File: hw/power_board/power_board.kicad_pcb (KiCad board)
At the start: 2 copper layers, 61 x 106.7 mm, 44 parts, among them P1 SIGNAL_IN, P10 SPINDLE_C_BLOCK, P11 POWER_IN, P12 SPINDLE_PWR_OUT, P2 SPINDLE_REALY, P3 SOFT_RELAY, P4 DIS_RELAY, P5 STEPPER_RELAY, P6 STOP_RELAY, P7 SPINDLE_RPWR_IN, P8 SOFT_RELAY_OUT, P9 DIS_RELAY_OUT, Q1 Q_NMOS_GDS, Q2 Q_NMOS_GDS, Q3 Q_NMOS_GDS, Q4 Q_NMOS_GDS, Q5 Q_NMOS_GDS

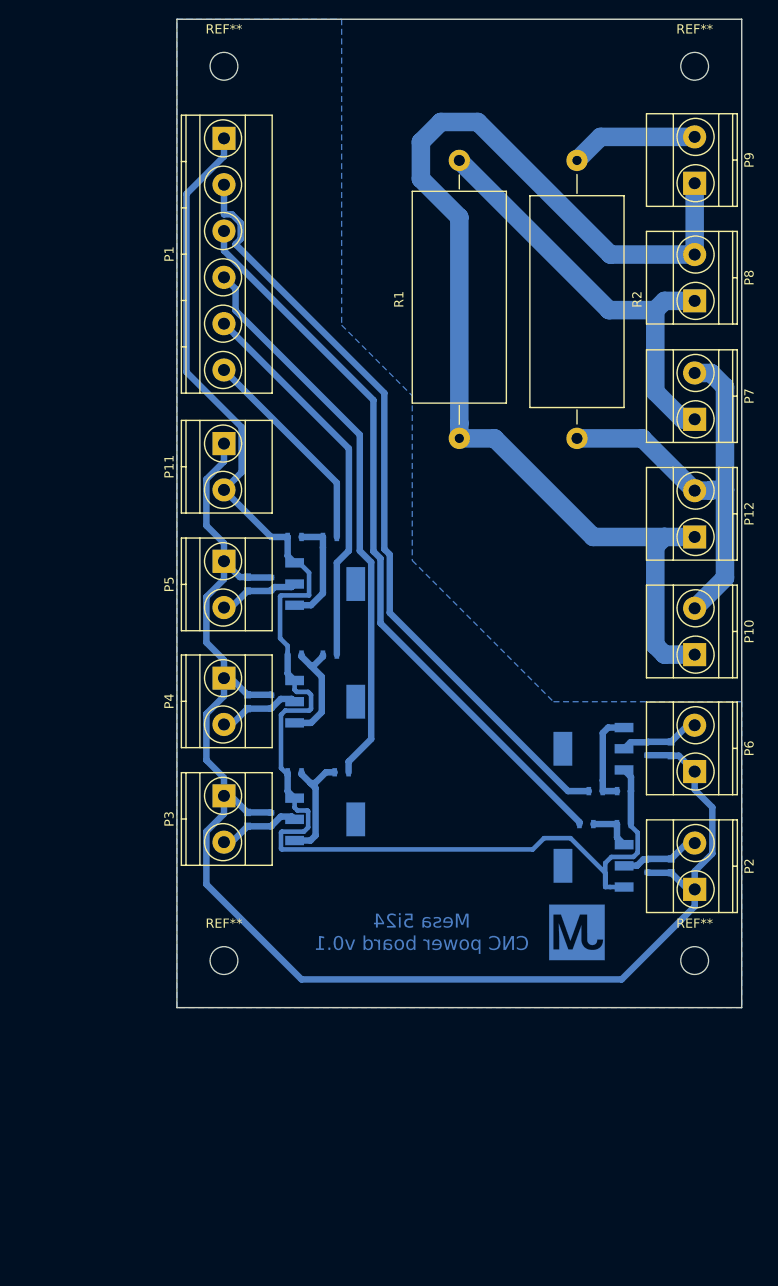
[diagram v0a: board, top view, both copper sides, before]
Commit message: Tweak power and breakout boards a little
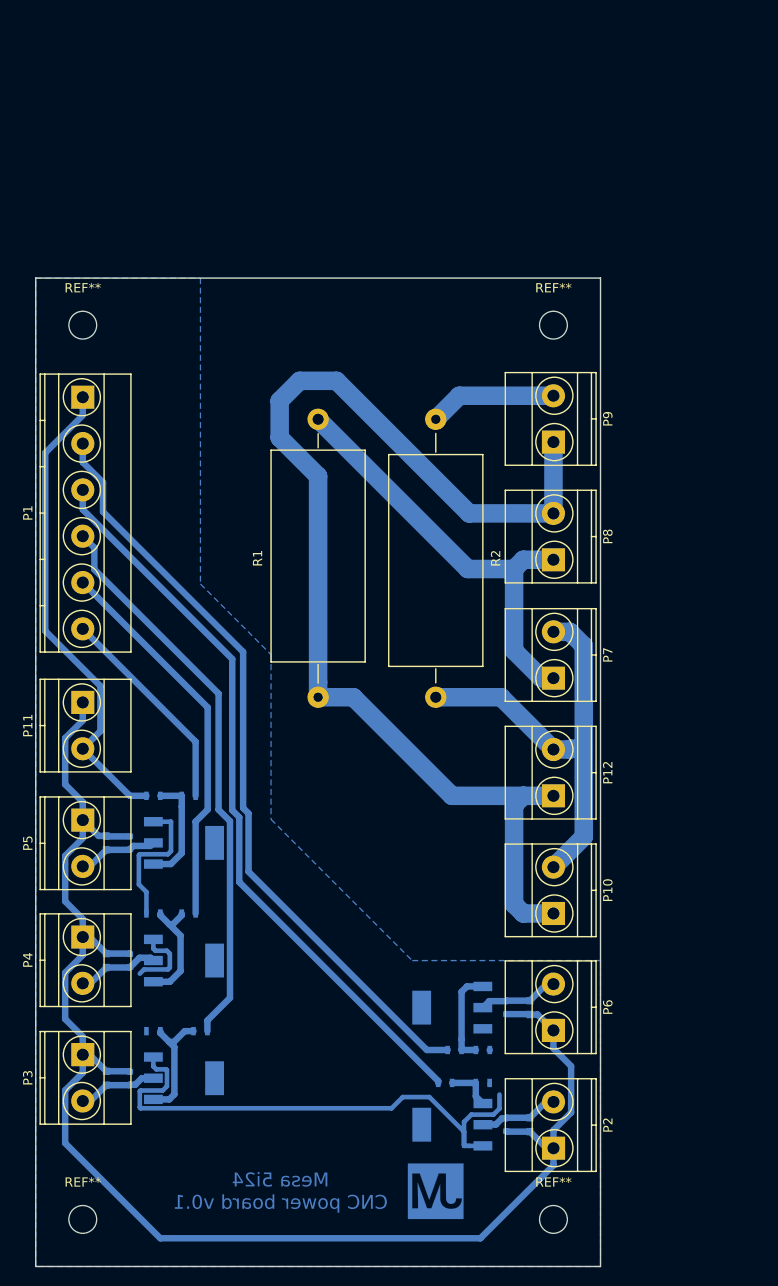
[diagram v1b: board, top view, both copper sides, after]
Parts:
- moved P2 31.8 mm to (127.0, 147.3)
- moved Q5 31.8 mm to (116.1, 132.1)
- moved C5 31.8 mm to (124.5, 132.1)
- moved D5 31.8 mm to (121.9, 132.1)
- moved REF** 31.8 mm to (127.0, 58.4)
- moved C3 31.8 mm to (78.7, 127.0)
- moved C4 31.8 mm to (78.7, 114.3)
- moved P10 31.8 mm to (127.0, 121.9)
- moved P12 31.8 mm to (127.0, 109.2)
- moved P6 31.8 mm to (127.0, 134.5)
- moved P7 31.8 mm to (127.0, 96.5)
- moved P8 31.8 mm to (127.0, 83.7)
- moved P9 31.8 mm to (127.0, 71.0)
- moved R1 31.8 mm to (101.6, 98.6)
- moved R10 31.8 mm to (83.8, 109.2)
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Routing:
- net GND: track 156.0 -> 134.2 mm
- net R_ESTOP: track 84.1 -> 83.1 mm
